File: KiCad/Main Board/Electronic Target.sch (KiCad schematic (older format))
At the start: 51 parts, among them J1 Conn_02x06_Odd_Even, J2 Conn_02x04_Odd_Even, U1 LM75AIMX_NOPB, U2 74LV8154, U3 LM339, U4 74HC74, U5 74HC00, U6 74LV8154, U7 74HC74, U8 NMA0505SC, X1 8M0

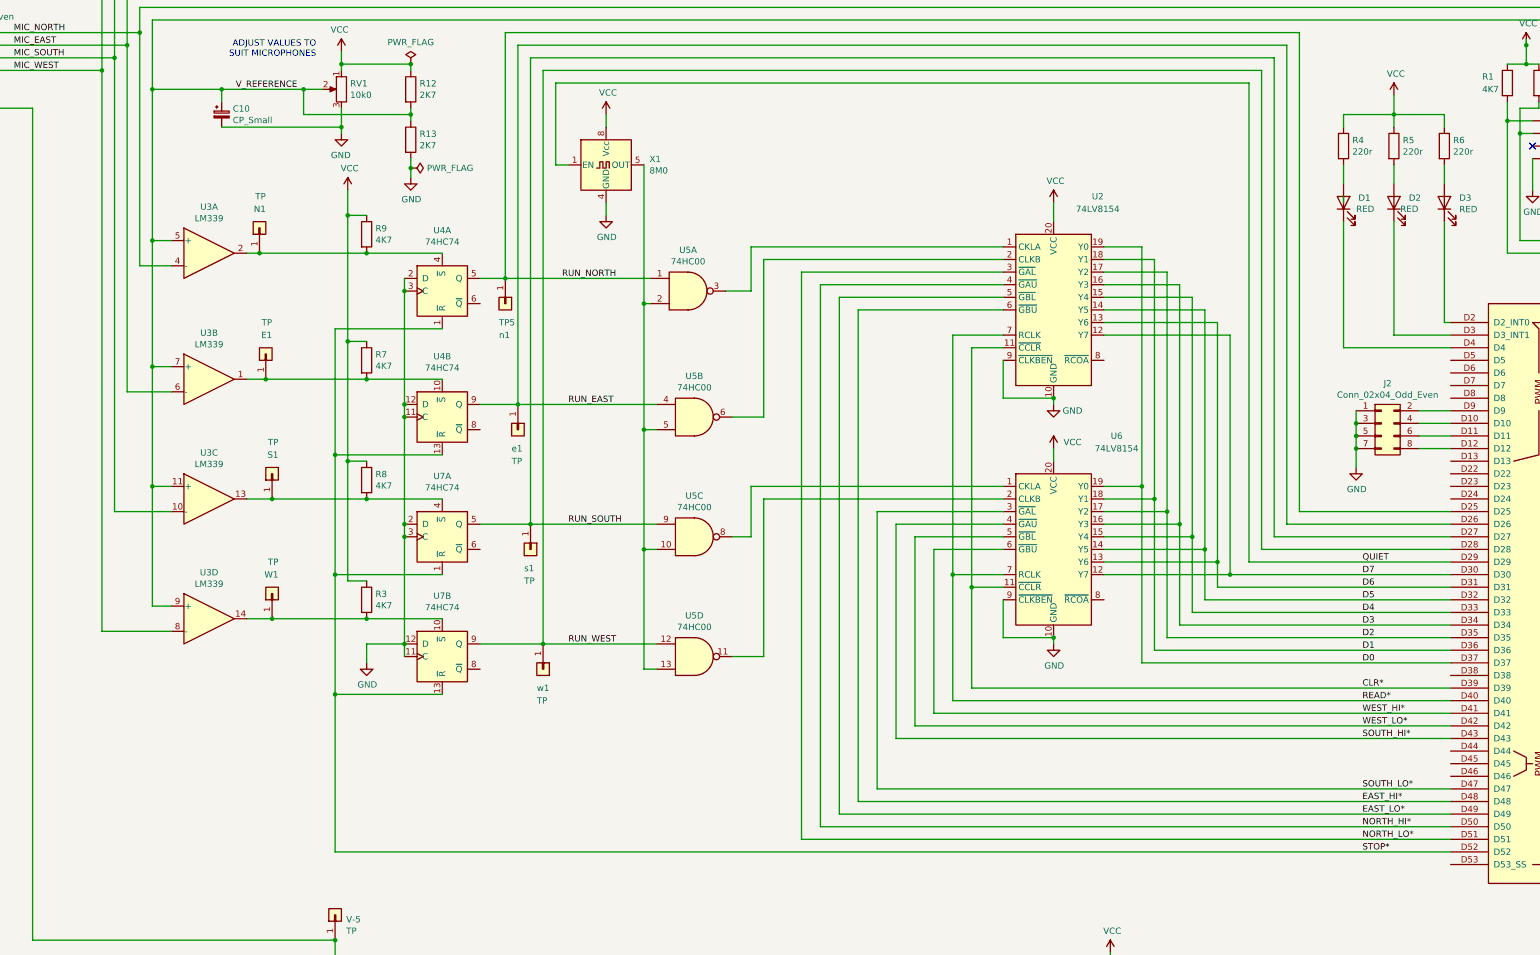
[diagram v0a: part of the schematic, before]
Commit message: In Progress for board debugging
Issue with East Sensor being investigated
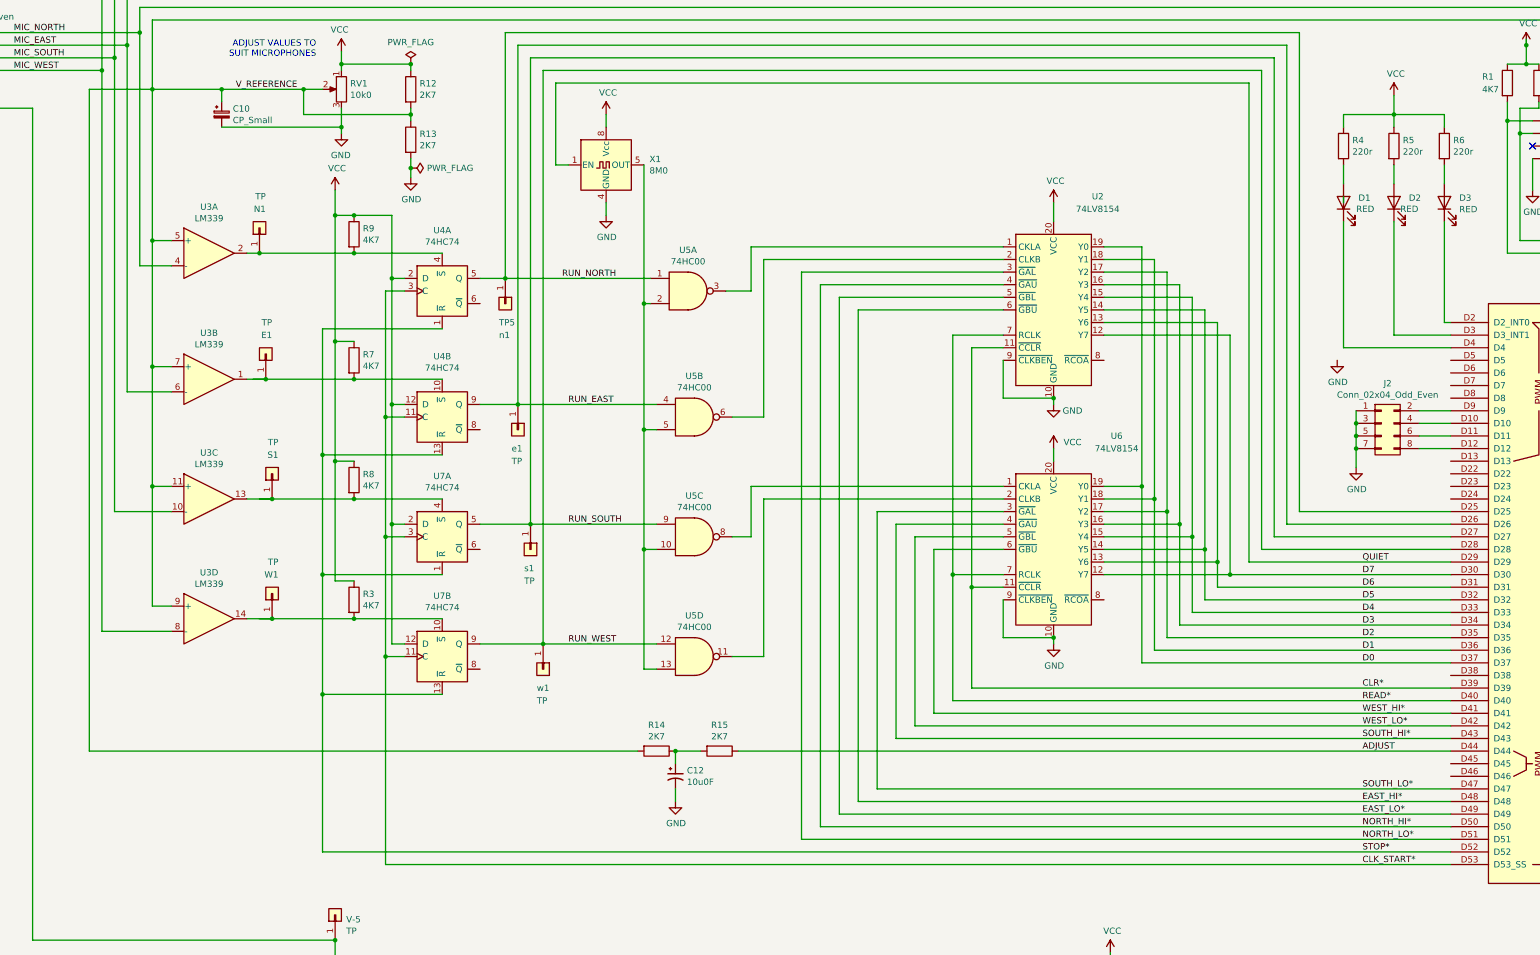
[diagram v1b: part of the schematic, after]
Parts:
- added C12: 10u0F, Resistor_SMD:R_0805_2012Metric, symbol Device:CP1_Small
- added R14, R15: 2K7, Resistor_SMD:R_0805_2012Metric, symbol Device:R
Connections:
- net GND: now also C12.2; no longer U4.11 (C), U4.12 (D), U4.2 (D), U4.3 (C), U7.11 (C), U7.12 (D), U7.2 (D), U7.3 (C)
- net VCC: now also U4.12 (D), U4.2 (D), U7.12 (D), U7.2 (D)
- net V_FB: now also R14.2
- net ADJUST: now reaches XA1.D44
- net ADJUST: now also R15.1
- net CLK_START*: now reaches XA1.D53 (D53_SS)
- net CLK_START*: now also U4.11 (C), U4.3 (C), U7.11 (C), U7.3 (C)
- new net: C12.1, R14.1, R15.2
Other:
- moved on the sheet: R3, R7, R8, R9
